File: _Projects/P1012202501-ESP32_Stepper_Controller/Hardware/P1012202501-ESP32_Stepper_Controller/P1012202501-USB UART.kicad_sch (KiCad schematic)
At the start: 8 parts, among them IC5 UCP2102C-A01-GQFN28

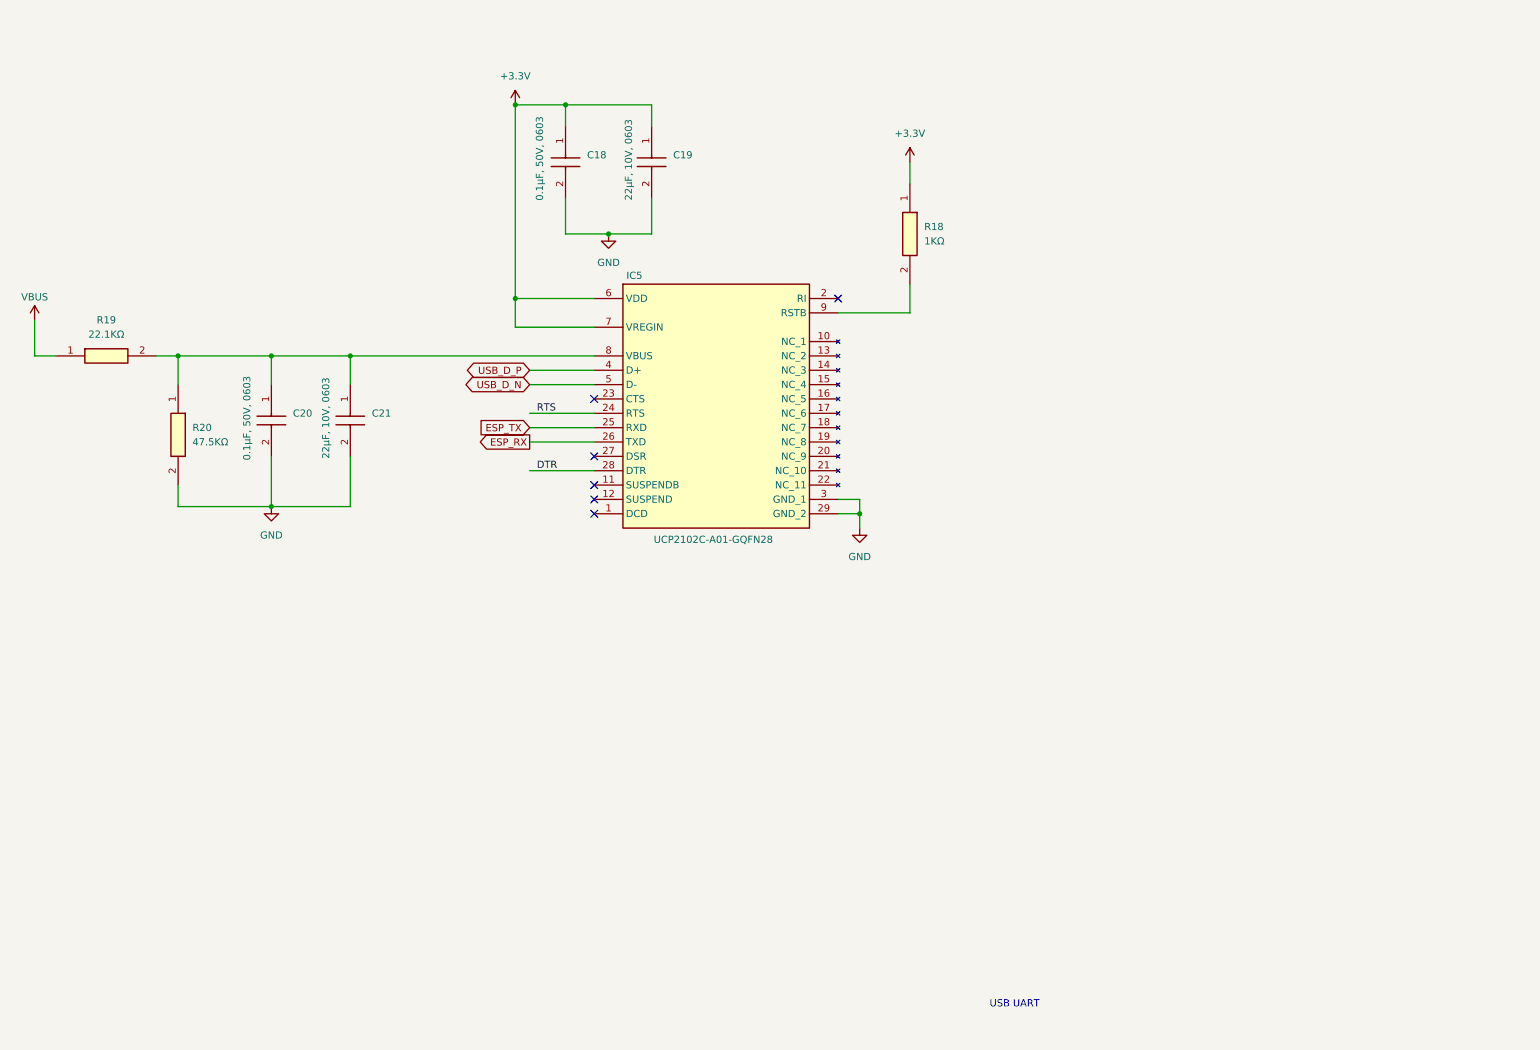
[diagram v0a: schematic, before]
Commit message: Added new content from stream.
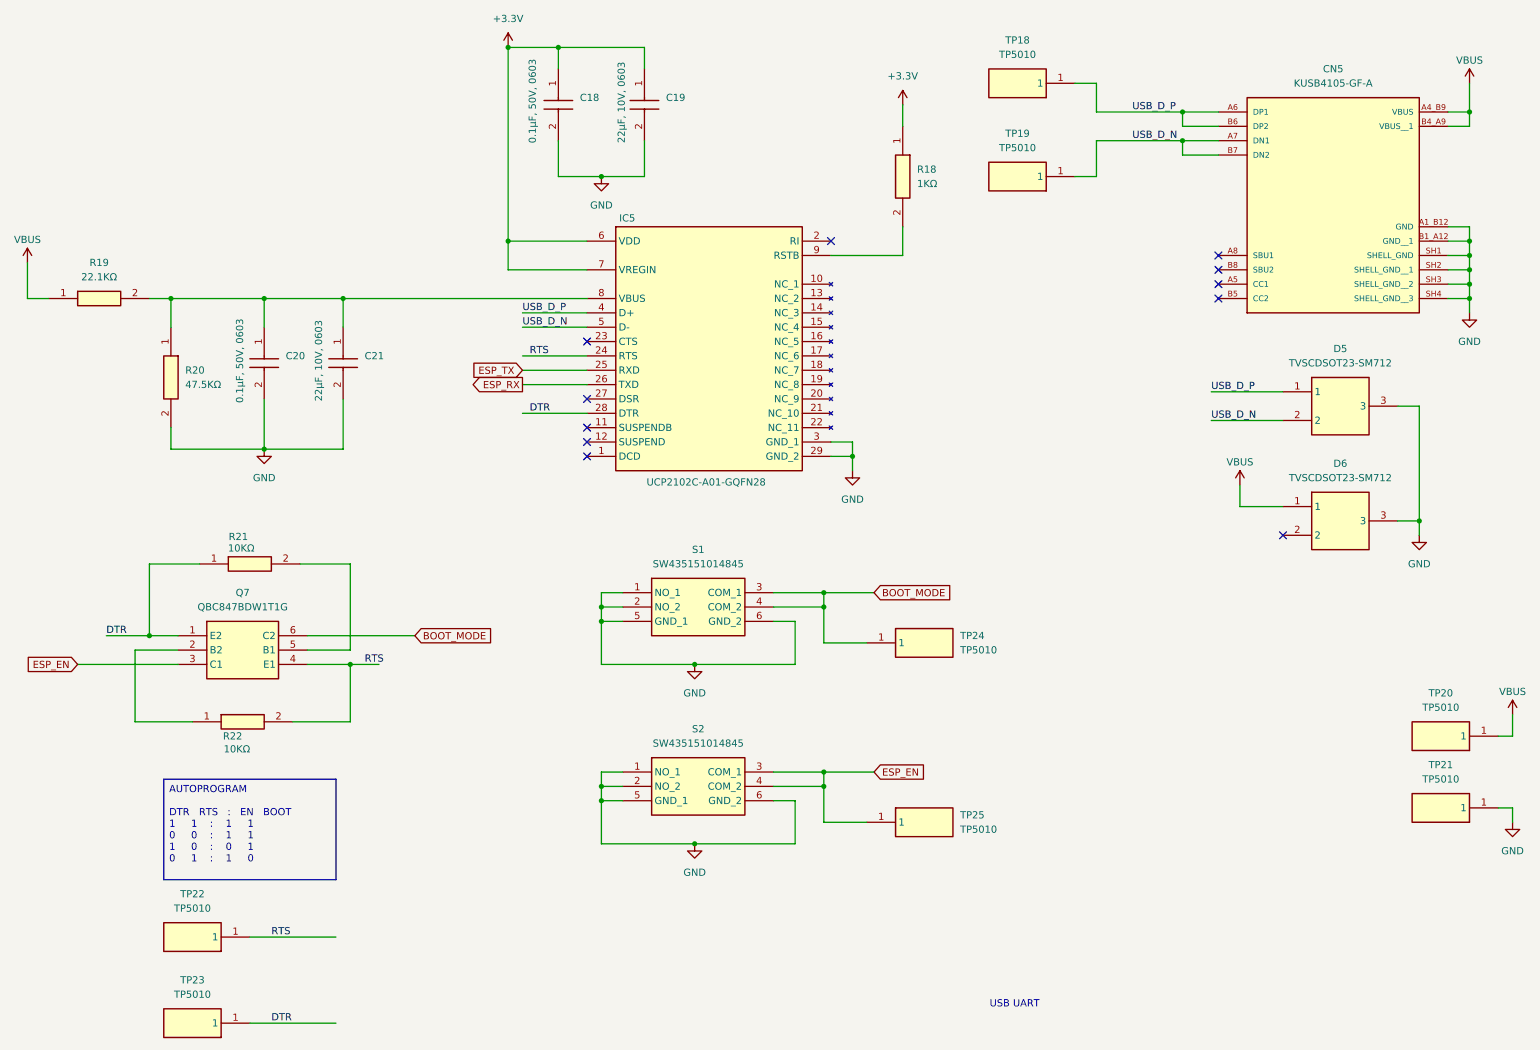
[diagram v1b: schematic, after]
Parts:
- added CN5: KUSB4105-GF-A, CONNECTORS:GCT_USB4105-GF-A, symbol CONNECTORS:KUSB4105-GF-A
- added D5, D6: TVSCDSOT23-SM712, COMPONENTS:SOT-23-3, symbol COMPONENTS:TVSCDSOT23-SM712
- added Q7: QBC847BDW1T1G, COMPONENTS:SC-70-6, symbol COMPONENTS:QBC847BDW1T1G
- added R21, R22: RC060310K2075AAA, COMPONENTS:RES-0603, symbol COMPONENTS:RC060310K2075AAA
- added S1, S2: SW435151014845, COMPONENTS:435151014845, symbol COMPONENTS:SW435151014845
- added TP18, TP19, TP20, TP21, TP22, TP23, TP24, TP25: TP5010, CONNECTORS:5010, symbol CONNECTORS:TP5010
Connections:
- net DTR: now also Q7.1 (E2), R21.1, TP23.1
- net GND: now also CN5.A1_B12 (GND), CN5.B1_A12 (GND__1), CN5.SH1 (SHELL_GND), CN5.SH2 (SHELL_GND__1), CN5.SH3 (SHELL_GND__2), CN5.SH4 (SHELL_GND__3), D5.3, D6.3, S1.1 (NO_1), S1.2 (NO_2), S1.5 (GND_1), S1.6 (GND_2), S2.1 (NO_1), S2.2 (NO_2), S2.5 (GND_1), S2.6 (GND_2), TP21.1
- net RTS: now also Q7.4 (E1), R22.2, TP22.1
- net USB_D_N: now also CN5.A7 (DN1), CN5.B7 (DN2), D5.2, TP19.1
- net USB_D_P: now also CN5.A6 (DP1), CN5.B6 (DP2), D5.1, TP18.1
- net VBUS: now also CN5.A4_B9 (VBUS), CN5.B4_A9 (VBUS__1), D6.1, TP20.1
- new net: Q7.2 (B2), R22.1
- new net: Q7.5 (B1), R21.2
- new net BOOT_MODE: Q7.6 (C2), S1.3 (COM_1), S1.4 (COM_2), TP24.1
- new net ESP_EN: Q7.3 (C1), S2.3 (COM_1), S2.4 (COM_2), TP25.1
- no-connect marks 6 -> 11
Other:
- moved on the sheet: C18, C19, C20, C21, IC5, R18, R19, R20
